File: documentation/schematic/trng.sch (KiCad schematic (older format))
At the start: 22 parts, among them Q1 BC320, U1 AD818

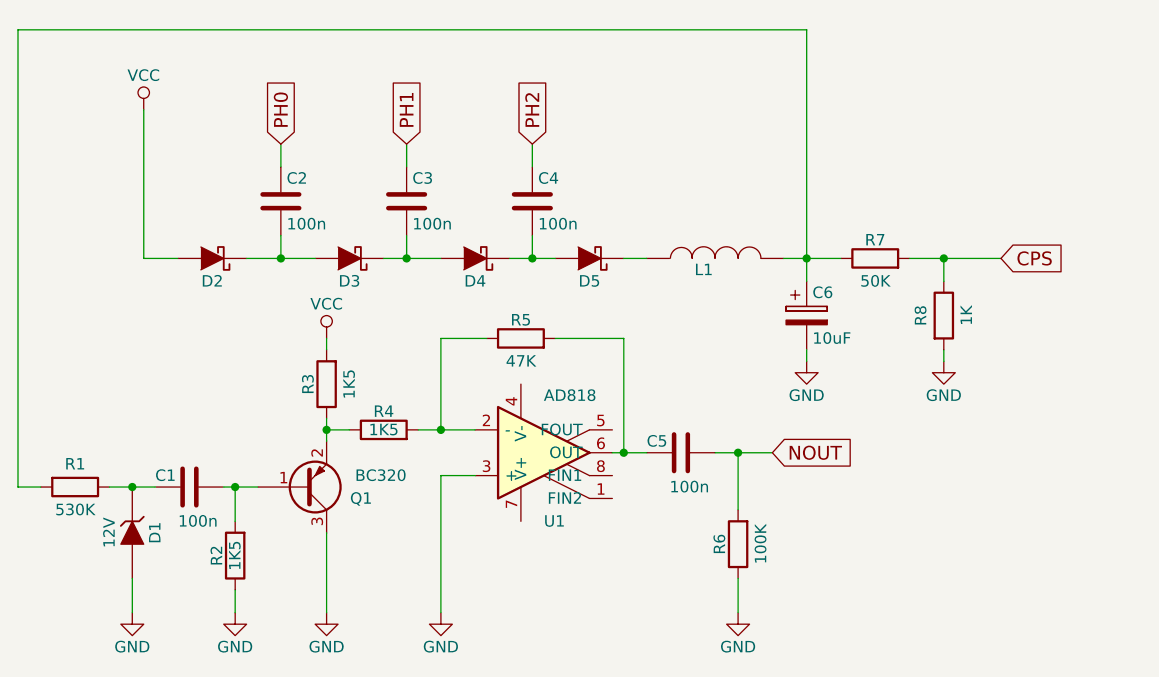
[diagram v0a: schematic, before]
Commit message: Update schematic
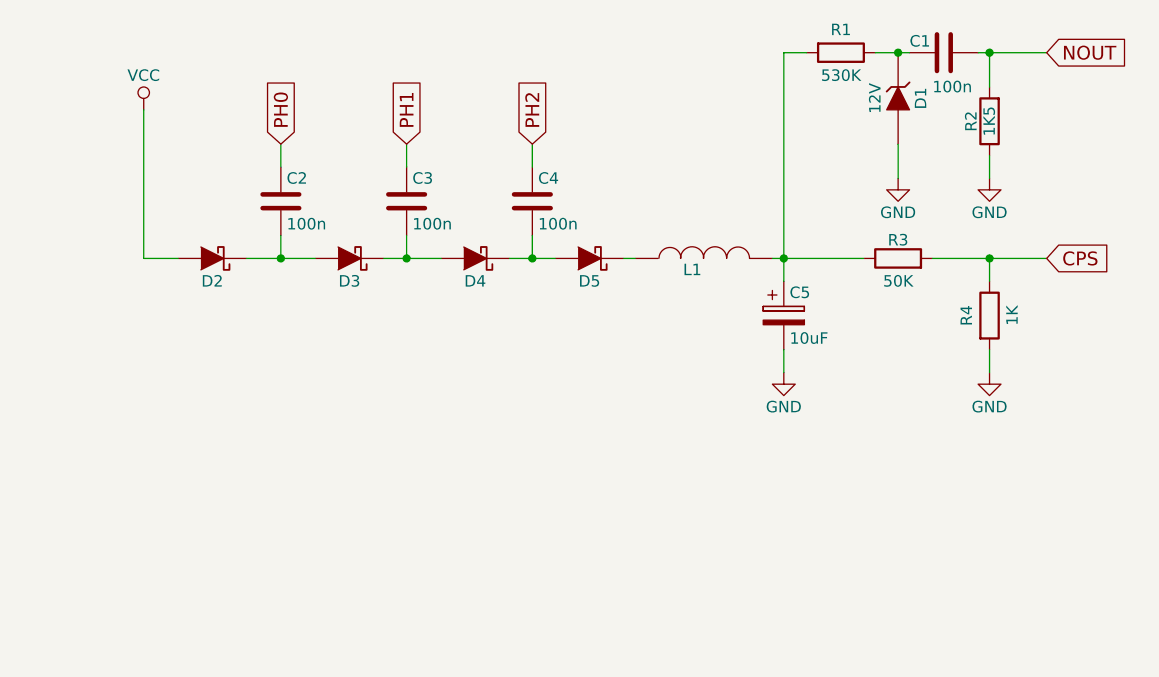
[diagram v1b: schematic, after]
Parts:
- removed C5: 100n, symbol C
- removed Q1: BC320, symbol Q_PNP_BEC
- removed R3, R4: 1K5, symbol R
- removed R5: 47K, symbol R
- removed R6: 100K, symbol R
- removed U1: AD818, symbol LM318N
- renumbered C6 to C5, R7 to R3, R8 to R4
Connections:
- net NOUT: now also C1.1, R2.2
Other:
- moved on the sheet: C1, C5, D1, L1, R1, R2, R3, R4
